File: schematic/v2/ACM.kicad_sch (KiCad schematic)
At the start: 12 parts, among them J1 FPGA I/O, J2 FPGA I/O, J8 FPGA I/O, J9 FPGA I/O

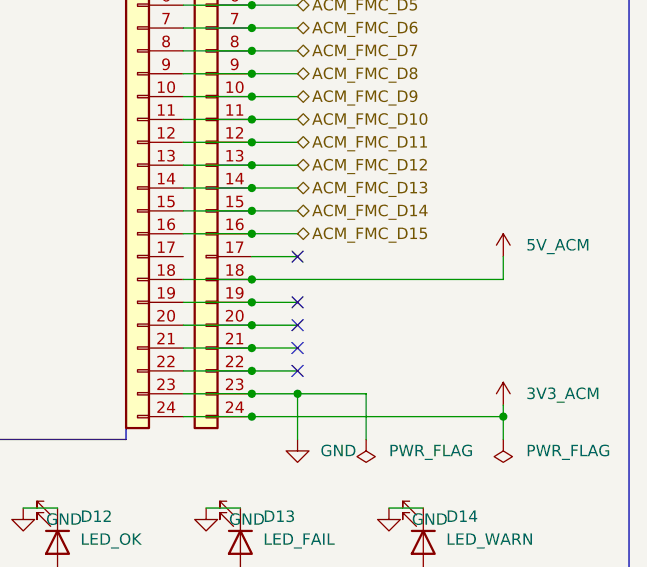
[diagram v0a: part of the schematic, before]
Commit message: no errors in the ERC!
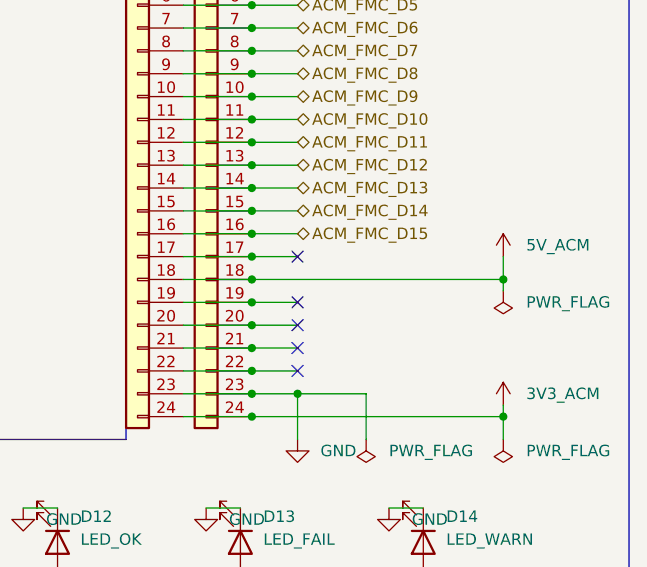
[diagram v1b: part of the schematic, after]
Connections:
- net at J9.17 (Pin_17): now also J2.17 (Pin_17)
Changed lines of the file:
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@@
 	)
 	(junction
+		(at 168.91 71.12)
+		(diameter 0)
+		(color 0 0 0 0)
+	)
+	(junction
 		(at 119.38 40.64)
 		(diameter 0)
@@
 	)
 	(junction
+		(at 196.85 73.66)
+		(diameter 0)
+		(color 0 0 0 0)
+	)
+	(junction
 		(at 196.85 88.9)
 		(diameter 0)
@@
 	(wire
 		(pts
+			(xy 196.85 74.93) (xy 196.85 73.66)
+		)
+		(stroke
+			(width 0)
+			(type default)
+		)
+	)
+	(wire
+		(pts
 			(xy 104.14 55.88) (xy 119.38 55.88)
 		)
@@
 	(wire
 		(pts
+			(xy 161.29 71.12) (xy 168.91 71.12)
+		)
+		(stroke
+			(width 0)
+			(type default)
+		)
+	)
+	(wire
+		(pts
 			(xy 119.38 38.1) (xy 127 38.1)
 		)
@@
 					(unit 1)
 				)
+			)
+		)
+	)
+	(symbol
+		(lib_id "power:PWR_FLAG")
+		(at 196.85 74.93 180)
+		(unit 1)
+		(exclude_from_sim no)
+		(in_bom yes)
+		(on_board yes)
+		(dnp no)
+		(fields_autoplaced yes)
+		(property "Reference" "#FLG01"
+			(at 196.85 76.835 0)
+			(effects
+				(font
+					(size 1.27 1.27)
+				)
+				(hide yes)
+			)
+		)
+		(property "Value" "PWR_FLAG"
+			(at 199.39 76.1999 0)
+			(effects
+				(font
+					(size 1.27 1.27)
+				)
+				(justify right)
+			)
+		)
+		(property "Footprint" ""
+			(at 196.85 74.93 0)
+			(effects
+				(font
+					(size 1.27 1.27)
+				)
+				(hide yes)
+			)
+		)
+		(property "Datasheet" "~"
+			(at 196.85 74.93 0)
+			(effects
+				(font
+					(size 1.27 1.27)
+				)
+				(hide yes)
+			)
+		)
+		(property "Description" "Special symbol for telling ERC where power comes from"
+			(at 196.85 74.93 0)
+			(effects
+				(font
+					(size 1.27 1.27)
+				)
+				(hide yes)
+			)
+		)
+		(pin "1"
+		)
+		(instances
+			(project "signalmesh"
+				(path "/fe7b15e9-f0ed-4338-9f03-dd7651dace13/c5977503-4ab2-47b6-bfc3-7f974cfcf6ea"
+					(reference "#FLG01")
+					(unit 1)
+				)
